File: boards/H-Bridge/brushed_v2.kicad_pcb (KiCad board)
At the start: 4 copper layers, 62 parts, among them IC1 ISO1042QDWVQ1, IC2 MIC4606-1YML-TR, IC3 AD8410AWBRZ-RL, IC4 TC1108-3.3VDBTR, J1 V+, J2 V-, J3 Motor-, J4 Motor+, J5 CANBus, J6 Encoder, J7 Prog_Header, J8 UART, J9 12V+, Q1 NTBLS4D0N15MC, Q2 NTBLS4D0N15MC, Q3 NTBLS4D0N15MC, Q4 NTBLS4D0N15MC, U1 STM32F103C8Tx, U2 LSF0102DCUR, U3 LSF0102DCUR

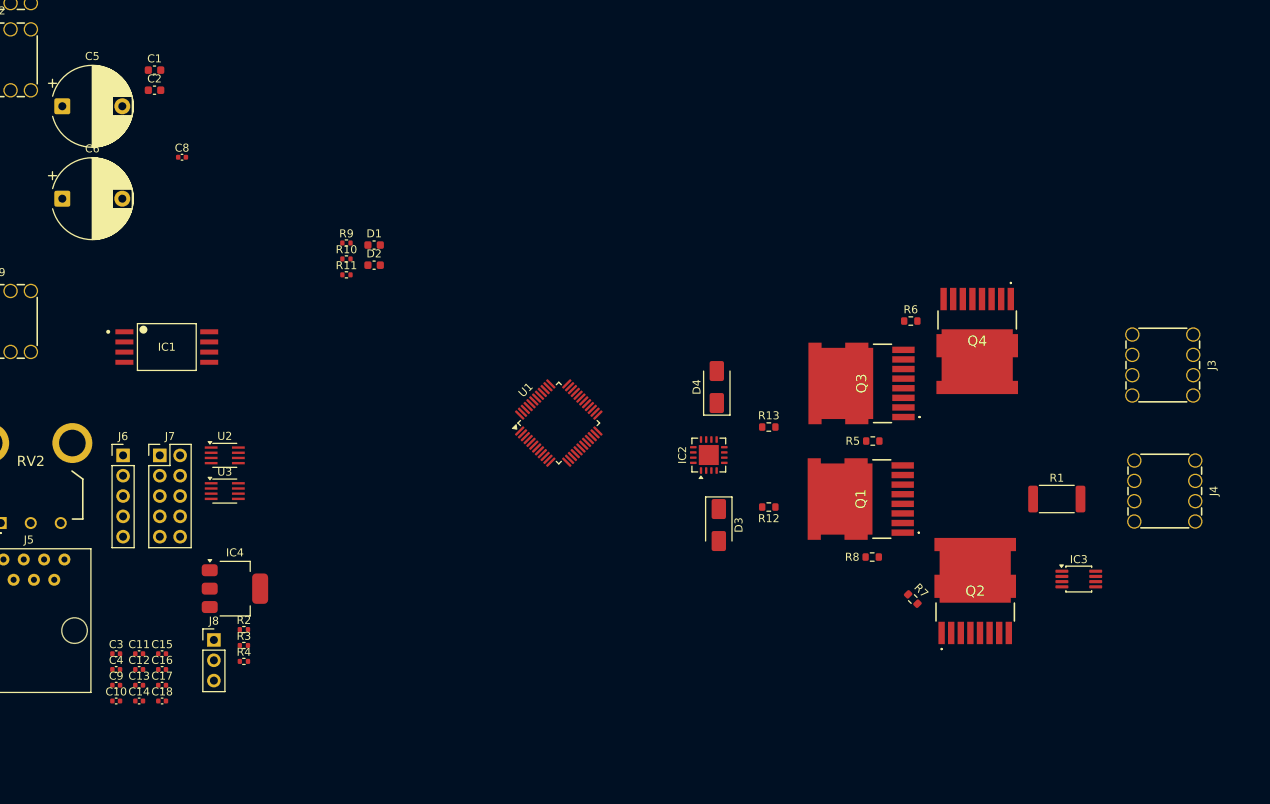
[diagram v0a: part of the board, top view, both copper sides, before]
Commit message: FET layout nearing completion
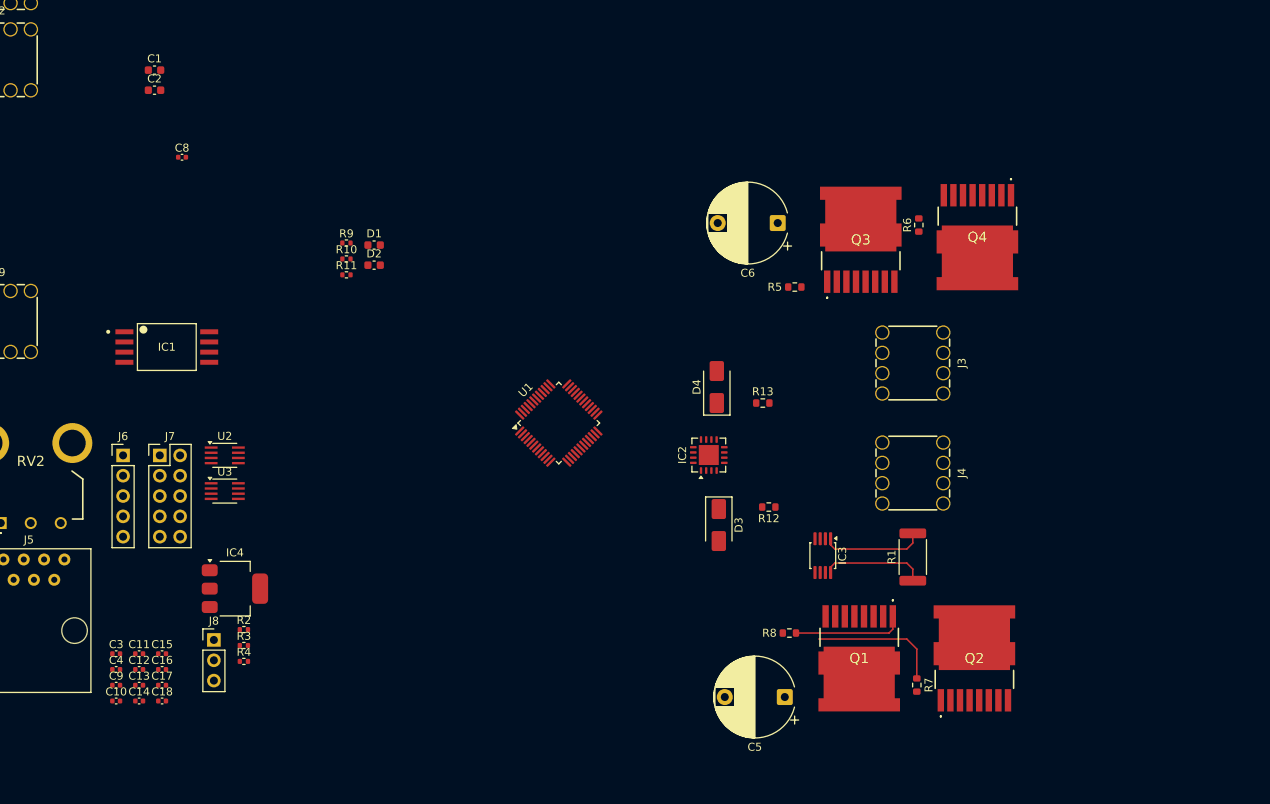
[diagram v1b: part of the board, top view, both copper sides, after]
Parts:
- moved C5 116.7 mm to (180.8, 140.5), turned to 180 degrees
- moved C6 89.5 mm to (179.9, 81.2), turned to 180 degrees
- moved IC3 32.1 mm to (185.5, 122.8), turned to -90 degrees
- moved J4 31.6 mm to (196.8, 112.5)
- moved J3 31.3 mm to (196.8, 98.8)
- moved R5 21.6 mm to (182.0, 89.2)
- moved Q1 19.9 mm to (190.1, 135.7), turned to 180 degrees
- moved R1 19.4 mm to (196.8, 123.0), turned to 90 degrees
- moved Q3 18.0 mm to (190.2, 83.3), turned to 0 degrees
- moved R8 14.0 mm to (181.3, 132.5)
- moved Q4 13.0 mm to (204.8, 83.0)
- moved R6 12.0 mm to (197.5, 81.5), turned to 90 degrees
- moved R7 10.8 mm to (197.2, 139.0), turned to 90 degrees
- moved Q2 8.42 mm to (204.4, 135.7)
- moved R13 3.09 mm to (178.0, 103.8)
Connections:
- J4 pad 1: /High Voltage&Sense/SHUNT+ -> /High Voltage&Sense/SHUNT-
- Q1 pad 1: /High Voltage&Sense/SHUNT- -> /High Voltage&Sense/SHUNT+
- Q1 pad 2: /High Voltage&Sense/SHUNT- -> /High Voltage&Sense/SHUNT+
- Q1 pad 3: /High Voltage&Sense/SHUNT- -> /High Voltage&Sense/SHUNT+
- Q1 pad 4: /High Voltage&Sense/SHUNT- -> /High Voltage&Sense/SHUNT+
- Q1 pad 5: /High Voltage&Sense/SHUNT- -> /High Voltage&Sense/SHUNT+
- Q1 pad 6: /High Voltage&Sense/SHUNT- -> /High Voltage&Sense/SHUNT+
- Q1 pad 7: /High Voltage&Sense/SHUNT- -> /High Voltage&Sense/SHUNT+
- Q2 pad 10: /High Voltage&Sense/SHUNT- -> /High Voltage&Sense/SHUNT+
- Q2 pad 11: /High Voltage&Sense/SHUNT- -> /High Voltage&Sense/SHUNT+
- Q2 pad 12: /High Voltage&Sense/SHUNT- -> /High Voltage&Sense/SHUNT+
- Q2 pad 13: /High Voltage&Sense/SHUNT- -> /High Voltage&Sense/SHUNT+
- Q2 pad 9: /High Voltage&Sense/SHUNT- -> /High Voltage&Sense/SHUNT+
- R1 pad 1: /High Voltage&Sense/SHUNT- -> /High Voltage&Sense/SHUNT+
- R1 pad 2: /High Voltage&Sense/SHUNT+ -> /High Voltage&Sense/SHUNT-
- R12 pad 1: /High Voltage&Sense/SHUNT- -> /High Voltage&Sense/SHUNT+
- U1 pad 26: /MCU&Low_Voltage/CHA_3.3 -> unconnected-(U1-PB13-Pad26)
- U1 pad 27: /MCU&Low_Voltage/CHB_3.3 -> unconnected-(U1-PB14-Pad27)
- U1 pad 42: unconnected-(U1-PB6-Pad42) -> /MCU&Low_Voltage/CHA_3.3
- U1 pad 43: unconnected-(U1-PB7-Pad43) -> /MCU&Low_Voltage/CHB_3.3
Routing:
- net Net-(IC2-ALO): track 0.00 -> 16.4 mm
- net /High Voltage&Sense/GATEA_HIGH: track 0.00 -> 13.9 mm
- net /High Voltage&Sense/SHUNT+: track 0.00 -> 12.9 mm
- net /High Voltage&Sense/SHUNT-: track 0.00 -> 12.8 mm
